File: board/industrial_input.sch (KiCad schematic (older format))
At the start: 3 parts

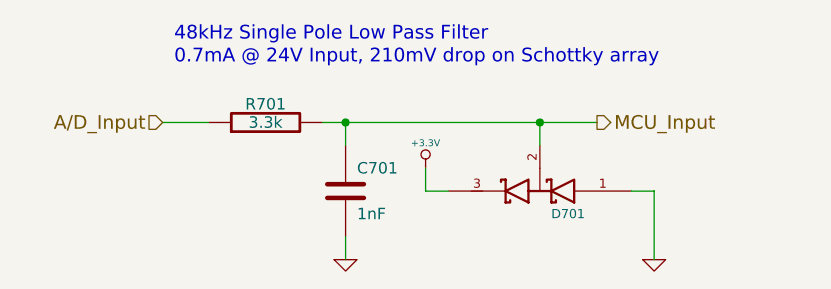
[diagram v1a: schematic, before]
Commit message: Layed out in general where stuff is going to be located.
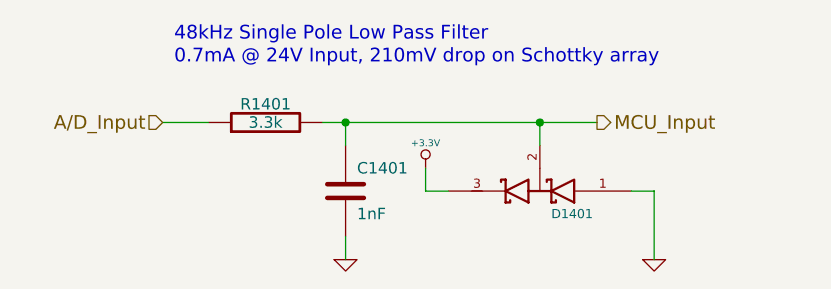
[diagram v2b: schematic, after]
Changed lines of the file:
@@
 AR Path="/52F88315/52E6DE87" Ref="R1301"  Part="1"
 AR Path="/52F88319/52E6DE87" Ref="R1401"  Part="1"
-F 0 "R701" V 5480 3950 50  0000 C CNN
+F 0 "R1401" V 5480 3950 50  0000 C CNN
 F 1 "3.3k" V 5400 3950 50  0000 C CNN
 F 2 "" H 5400 3950 60  0000 C CNN
@@
 AR Path="/52F88315/52E6DEAB" Ref="C1301"  Part="1"
 AR Path="/52F88319/52E6DEAB" Ref="C1401"  Part="1"
-F 0 "C701" H 5800 4350 50  0000 L CNN
+F 0 "C1401" H 5800 4350 50  0000 L CNN
 F 1 "1nF" H 5800 4150 50  0000 L CNN
 F 2 "" H 5750 4250 60  0000 C CNN
@@
 $EndComp
 $Comp
-L GND #PWR0140
+L GND #PWR702
 U 1 1 52E6DEC4
 P 5750 4550
-AR Path="/52F84966/52E6DEC4" Ref="#PWR0140"  Part="1"
-AR Path="/52F85705/52E6DEC4" Ref="#PWR0143"  Part="1"
-AR Path="/52F85B83/52E6DEC4" Ref="#PWR0146"  Part="1"
-AR Path="/52F85B87/52E6DEC4" Ref="#PWR0149"  Part="1"
-AR Path="/52F8830D/52E6DEC4" Ref="#PWR0152"  Part="1"
-AR Path="/52F88311/52E6DEC4" Ref="#PWR0155"  Part="1"
-AR Path="/52F88315/52E6DEC4" Ref="#PWR0158"  Part="1"
-AR Path="/52F88319/52E6DEC4" Ref="#PWR0161"  Part="1"
-F 0 "#PWR0161" H 5750 4550 30  0001 C CNN
+AR Path="/52F84966/52E6DEC4" Ref="#PWR702"  Part="1"
+AR Path="/52F85705/52E6DEC4" Ref="#PWR802"  Part="1"
+AR Path="/52F85B83/52E6DEC4" Ref="#PWR902"  Part="1"
+AR Path="/52F85B87/52E6DEC4" Ref="#PWR1002"  Part="1"
+AR Path="/52F8830D/52E6DEC4" Ref="#PWR1102"  Part="1"
+AR Path="/52F88311/52E6DEC4" Ref="#PWR1202"  Part="1"
+AR Path="/52F88315/52E6DEC4" Ref="#PWR1302"  Part="1"
+AR Path="/52F88319/52E6DEC4" Ref="#PWR1402"  Part="1"
+F 0 "#PWR1402" H 5750 4550 30  0001 C CNN
 F 1 "GND" H 5750 4480 30  0001 C CNN
 F 2 "" H 5750 4550 60  0000 C CNN
@@
 $EndComp
 $Comp
-L GND #PWR0141
+L GND #PWR703
 U 1 1 52E6DFEB
 P 7100 4550
-AR Path="/52F84966/52E6DFEB" Ref="#PWR0141"  Part="1"
-AR Path="/52F85705/52E6DFEB" Ref="#PWR0144"  Part="1"
-AR Path="/52F85B83/52E6DFEB" Ref="#PWR0147"  Part="1"
-AR Path="/52F85B87/52E6DFEB" Ref="#PWR0150"  Part="1"
-AR Path="/52F8830D/52E6DFEB" Ref="#PWR0153"  Part="1"
-AR Path="/52F88311/52E6DFEB" Ref="#PWR0156"  Part="1"
-AR Path="/52F88315/52E6DFEB" Ref="#PWR0159"  Part="1"
-AR Path="/52F88319/52E6DFEB" Ref="#PWR0162"  Part="1"
-F 0 "#PWR0162" H 7100 4550 30  0001 C CNN
+AR Path="/52F84966/52E6DFEB" Ref="#PWR703"  Part="1"
+AR Path="/52F85705/52E6DFEB" Ref="#PWR803"  Part="1"
+AR Path="/52F85B83/52E6DFEB" Ref="#PWR903"  Part="1"
+AR Path="/52F85B87/52E6DFEB" Ref="#PWR1003"  Part="1"
+AR Path="/52F8830D/52E6DFEB" Ref="#PWR1103"  Part="1"
+AR Path="/52F88311/52E6DFEB" Ref="#PWR1203"  Part="1"
+AR Path="/52F88315/52E6DFEB" Ref="#PWR1303"  Part="1"
+AR Path="/52F88319/52E6DFEB" Ref="#PWR1403"  Part="1"
+F 0 "#PWR1403" H 7100 4550 30  0001 C CNN
 F 1 "GND" H 7100 4480 30  0001 C CNN
 F 2 "" H 7100 4550 60  0000 C CNN
@@
 AR Path="/52F88315/52E6E5BB" Ref="D1301"  Part="1"
 AR Path="/52F88319/52E6E5BB" Ref="D1401"  Part="1"
-F 0 "D701" H 6550 4350 40  0000 R CNN
+F 0 "D1401" H 6550 4350 40  0000 R CNN
 F 1 "1SS295" H 6550 4100 40  0001 R CNN
 F 2 "" H 6600 4250 60  0000 C CNN
@@
 0.7mA @ 24V Input, 210mV drop on Schottky array
 $Comp
-L +3.3V #PWR0142
+L +3.3V #PWR701
 U 1 1 5301839B
 P 6100 4150
-AR Path="/52F84966/5301839B" Ref="#PWR0142"  Part="1"
-AR Path="/52F85705/5301839B" Ref="#PWR0145"  Part="1"
-AR Path="/52F85B83/5301839B" Ref="#PWR0148"  Part="1"
-AR Path="/52F85B87/5301839B" Ref="#PWR0151"  Part="1"
-AR Path="/52F8830D/5301839B" Ref="#PWR0154"  Part="1"
-AR Path="/52F88311/5301839B" Ref="#PWR0157"  Part="1"
-AR Path="/52F88315/5301839B" Ref="#PWR0160"  Part="1"
-AR Path="/52F88319/5301839B" Ref="#PWR0163"  Part="1"
-F 0 "#PWR0163" H 6100 4110 30  0001 C CNN
+AR Path="/52F84966/5301839B" Ref="#PWR701"  Part="1"
+AR Path="/52F85705/5301839B" Ref="#PWR801"  Part="1"
+AR Path="/52F85B83/5301839B" Ref="#PWR901"  Part="1"
+AR Path="/52F85B87/5301839B" Ref="#PWR1001"  Part="1"
+AR Path="/52F8830D/5301839B" Ref="#PWR1101"  Part="1"
+AR Path="/52F88311/5301839B" Ref="#PWR1201"  Part="1"
+AR Path="/52F88315/5301839B" Ref="#PWR1301"  Part="1"
+AR Path="/52F88319/5301839B" Ref="#PWR1401"  Part="1"
+F 0 "#PWR1401" H 6100 4110 30  0001 C CNN
 F 1 "+3.3V" H 6100 4260 30  0000 C CNN
 F 2 "" H 6100 4150 60  0000 C CNN
